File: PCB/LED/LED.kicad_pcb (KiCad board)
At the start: 2 copper layers, 70 x 70 mm, 33 parts, among them J1 Reset, J2 Wago, J3 TC2030-USB-NL-DS, J5 USB-C-Socket-H, SW1 Button, U1 ICS43434_MEMS_Mic, U6 ESP32-S3-MINI-1, U7 MD8942

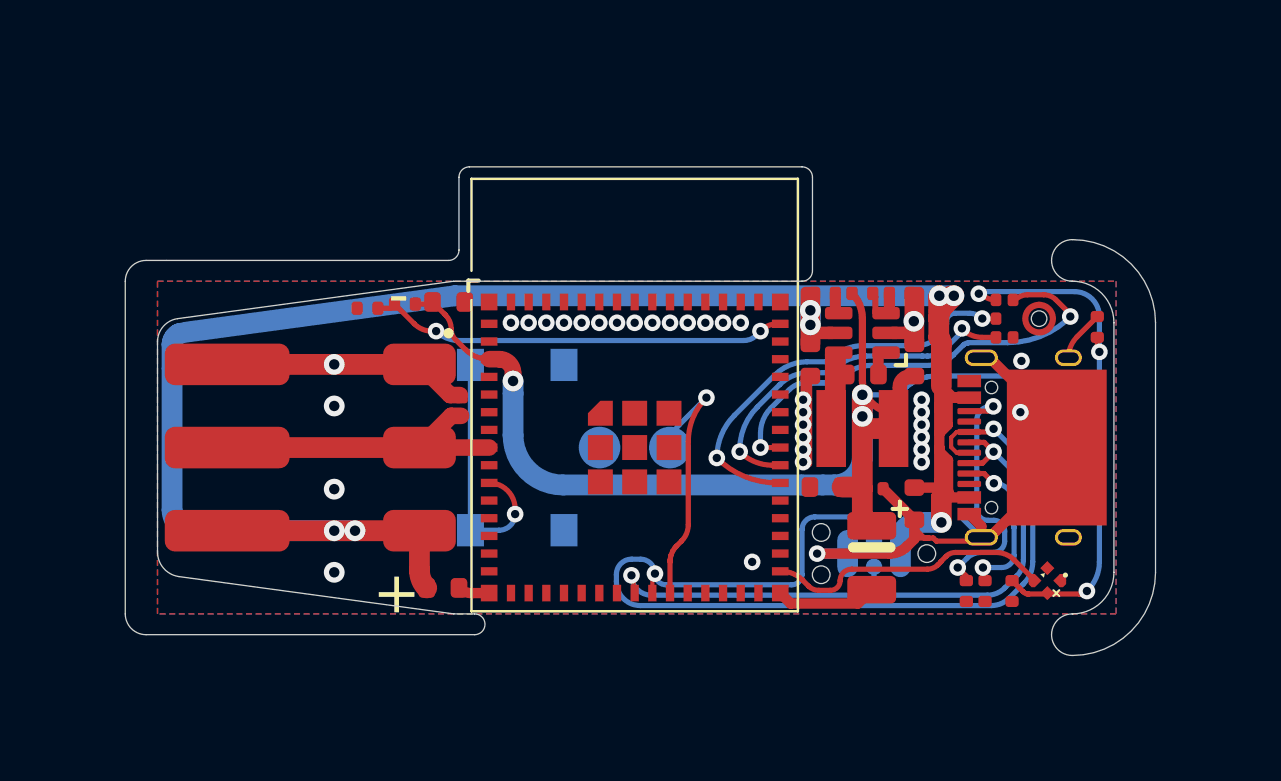
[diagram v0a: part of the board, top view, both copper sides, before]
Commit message: ADC
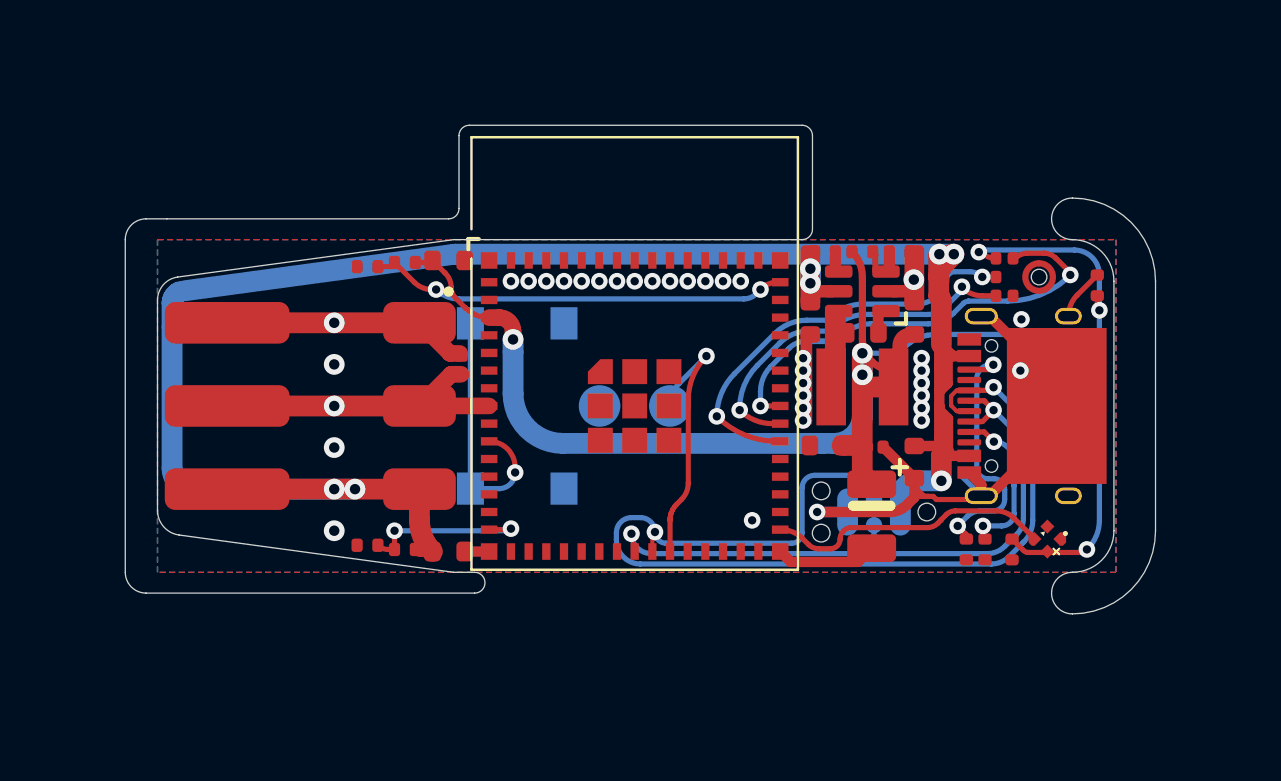
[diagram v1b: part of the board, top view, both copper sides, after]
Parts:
- added R1: 124K, RevK:R_0402, F.Cu at (87.4, 106.9)
- added R3: 10K, RevK:R_0402, F.Cu at (85.6, 106.7)
- moved C1 2.00 mm to (109.8, 105.3)
- moved C10 2.00 mm to (106.9, 95.8)
- moved C11 2.00 mm to (111.9, 95.8)
- moved C12 2.00 mm to (109.4, 96.5)
- moved C2 2.00 mm to (109.9, 102.0)
- moved C3 2.00 mm to (107.7, 101.9)
- moved C4 2.00 mm to (116.6, 106.9)
- moved C5 2.00 mm to (111.9, 102.7)
- moved C7 2.00 mm to (89.5, 93.0)
- moved C8 2.00 mm to (120.7, 94.2)
- moved C9 2.00 mm to (85.6, 93.3)
- moved D1 2.00 mm to (118.3, 106.4)
- moved D2 2.00 mm to (90.1, 98.0)
- moved J1 2.00 mm to (98.5, 100.0)
- moved J2 2.00 mm to (83.5, 100.0)
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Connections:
- U6 pad 15: unconnected-(U6-GPIO11-Pad15) -> ADC
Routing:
- net ADC: track 0.00 -> 8.44 mm, vias 0 -> 2
- net DC: track 97.4 -> 98.6 mm
- net LED: vias 0 -> 1
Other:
- board text added: "11"
